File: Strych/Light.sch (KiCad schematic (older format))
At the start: 18 parts

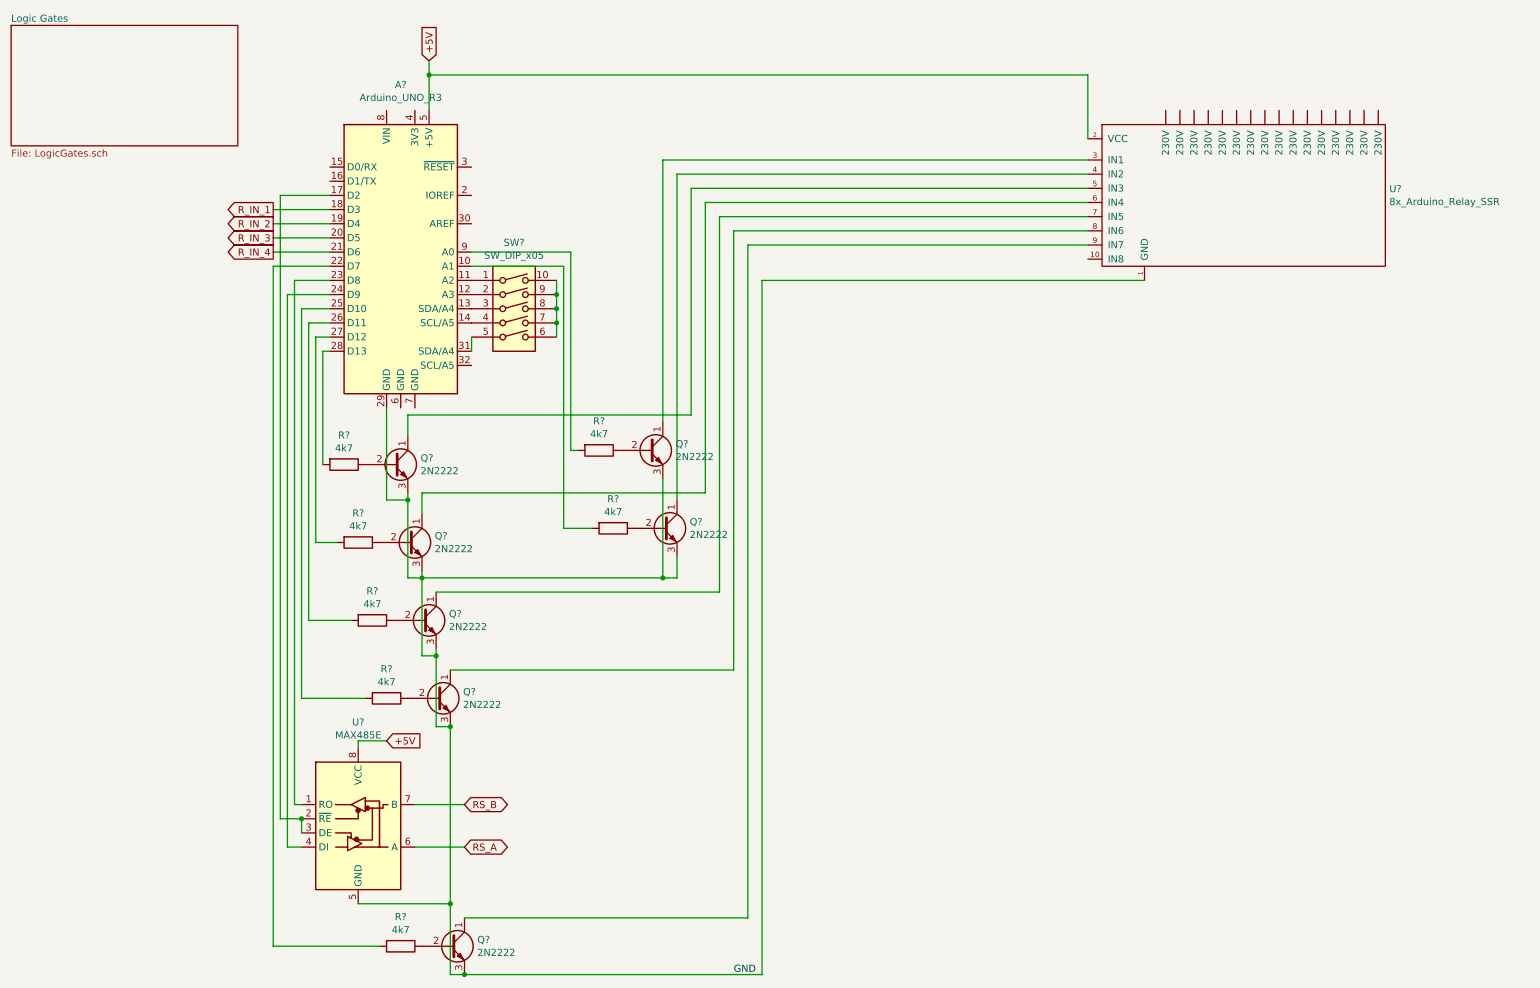
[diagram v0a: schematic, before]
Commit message: Delete lights
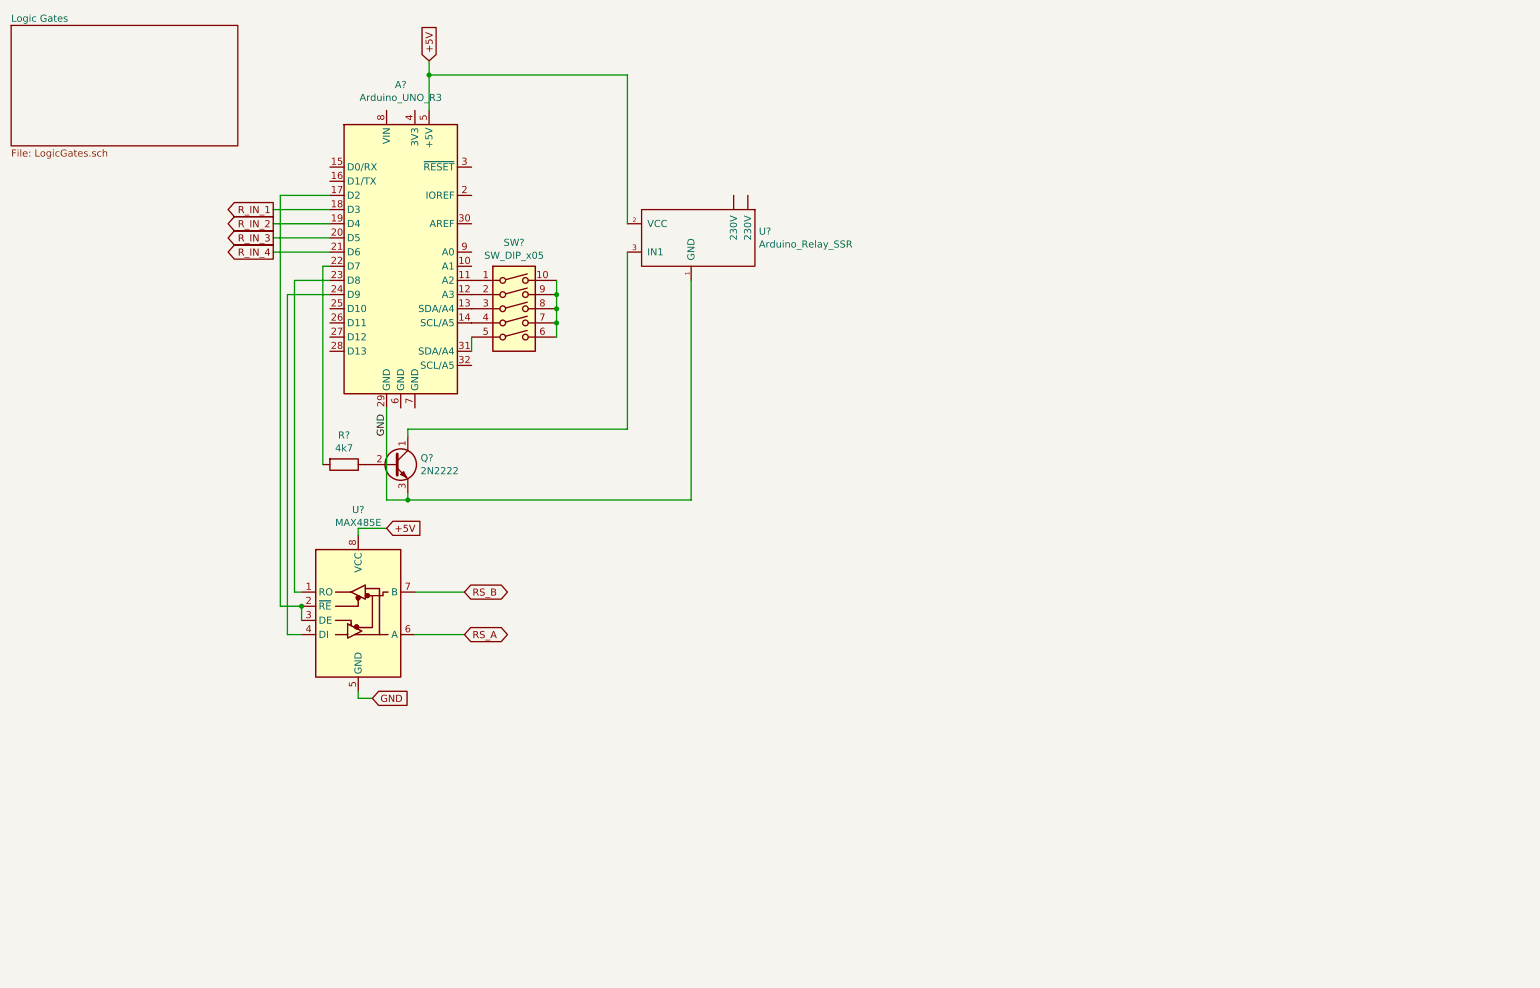
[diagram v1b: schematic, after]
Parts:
- removed Q? (x6): 2N2222, Package_TO_SOT_THT:TO-92_Inline, symbol Transistor_BJT:BC237
- removed R? (x6): 4k7, symbol Device:R
- removed U?: 8x_Arduino_Relay_SSR, symbol Arduino_Relay:8x_Arduino_Relay_SSR
- added U?: Arduino_Relay_SSR, symbol Arduino_Relay:Arduino_Relay_SSR
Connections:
- net +5V: now also U?.2 (VCC)
- net GND: now also U?.1 (GND)
- net at Q?.1 (C): now also U?.3 (IN1)
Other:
- moved on the sheet: Q?, R?, U?
